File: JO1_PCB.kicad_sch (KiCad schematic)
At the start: 1 part, among them U2 module_mpu6050

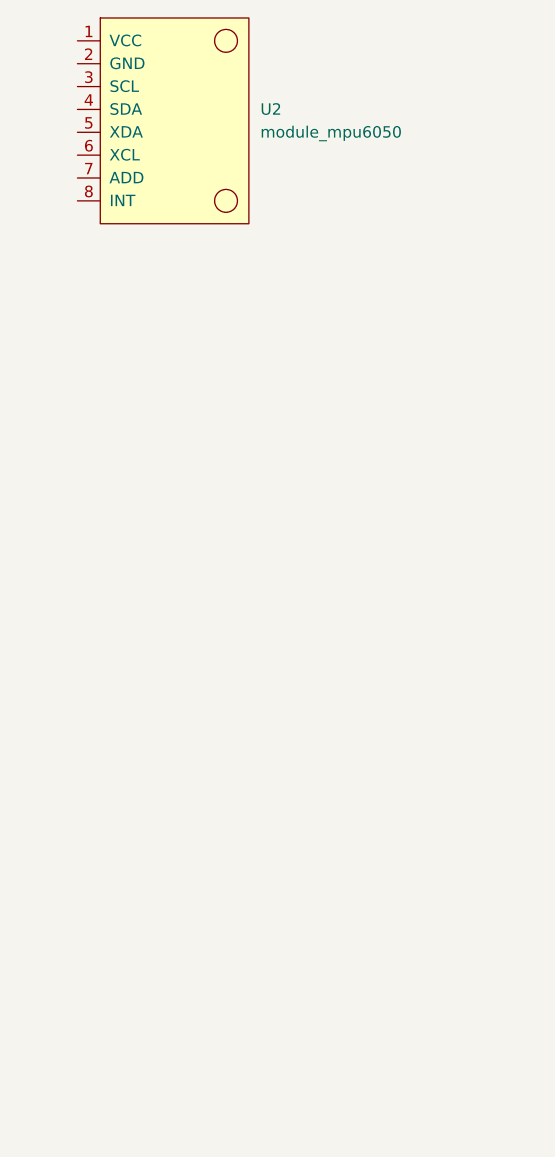
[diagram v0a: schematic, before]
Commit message: CN7 header done
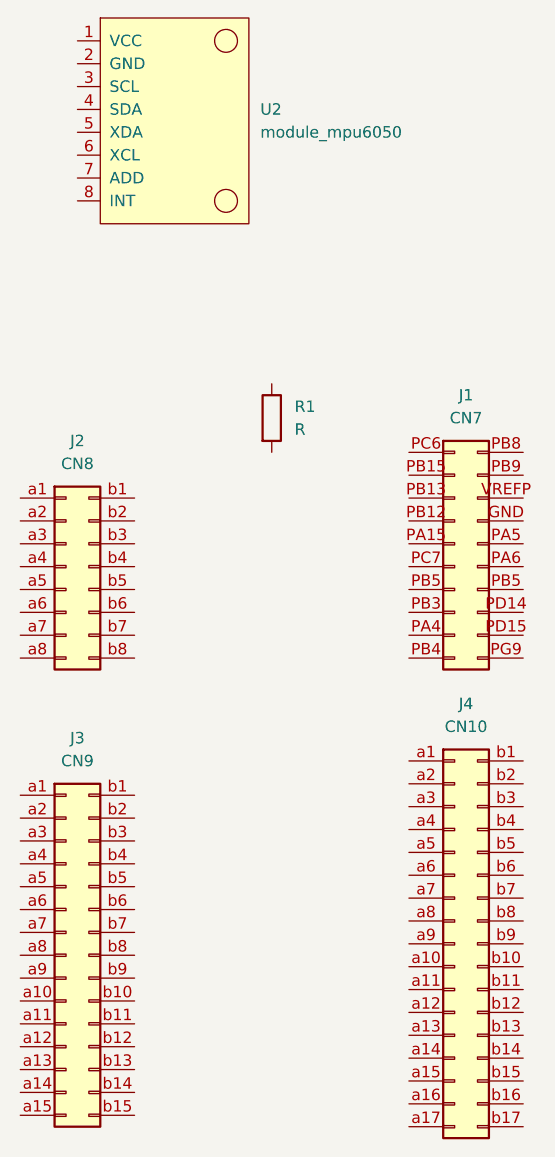
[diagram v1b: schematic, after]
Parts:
- added J1: CN7, Connector_PinHeader_2.54mm:PinHeader_2x10_P2.54mm_Vertical, symbol Connector_Generic:Conn_02x10_Row_Letter_First
- added J2: CN8, Connector_PinHeader_2.54mm:PinHeader_2x08_P2.54mm_Vertical, symbol Connector_Generic:Conn_02x08_Row_Letter_First
- added J3: CN9, Connector_PinHeader_2.54mm:PinHeader_2x15_P2.54mm_Vertical, symbol Connector_Generic:Conn_02x15_Row_Letter_First
- added J4: CN10, Connector_PinHeader_2.54mm:PinHeader_2x17_P2.54mm_Vertical, symbol Connector_Generic:Conn_02x17_Row_Letter_First
- added R1: R, Resistor_THT:R_Axial_DIN0411_L9.9mm_D3.6mm_P15.24mm_Horizontal, symbol Device:R
